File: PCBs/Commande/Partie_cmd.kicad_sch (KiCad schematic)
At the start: 74 parts, among them J1 Barrel_Jack, J10 Conn_01x02, J2 Conn_01x04_Socket, J3 Conn_01x04_Socket, J4 Conn_01x15, J6 Conn_01x04, J7 Conn_01x04, J9 Conn_01x02, U1 ESP32-S3-DEVKITC-1-N8R2, U2 BU18SD5WG-TL, U3 BU33SD5WG-TR, U4 XL1509-5.0

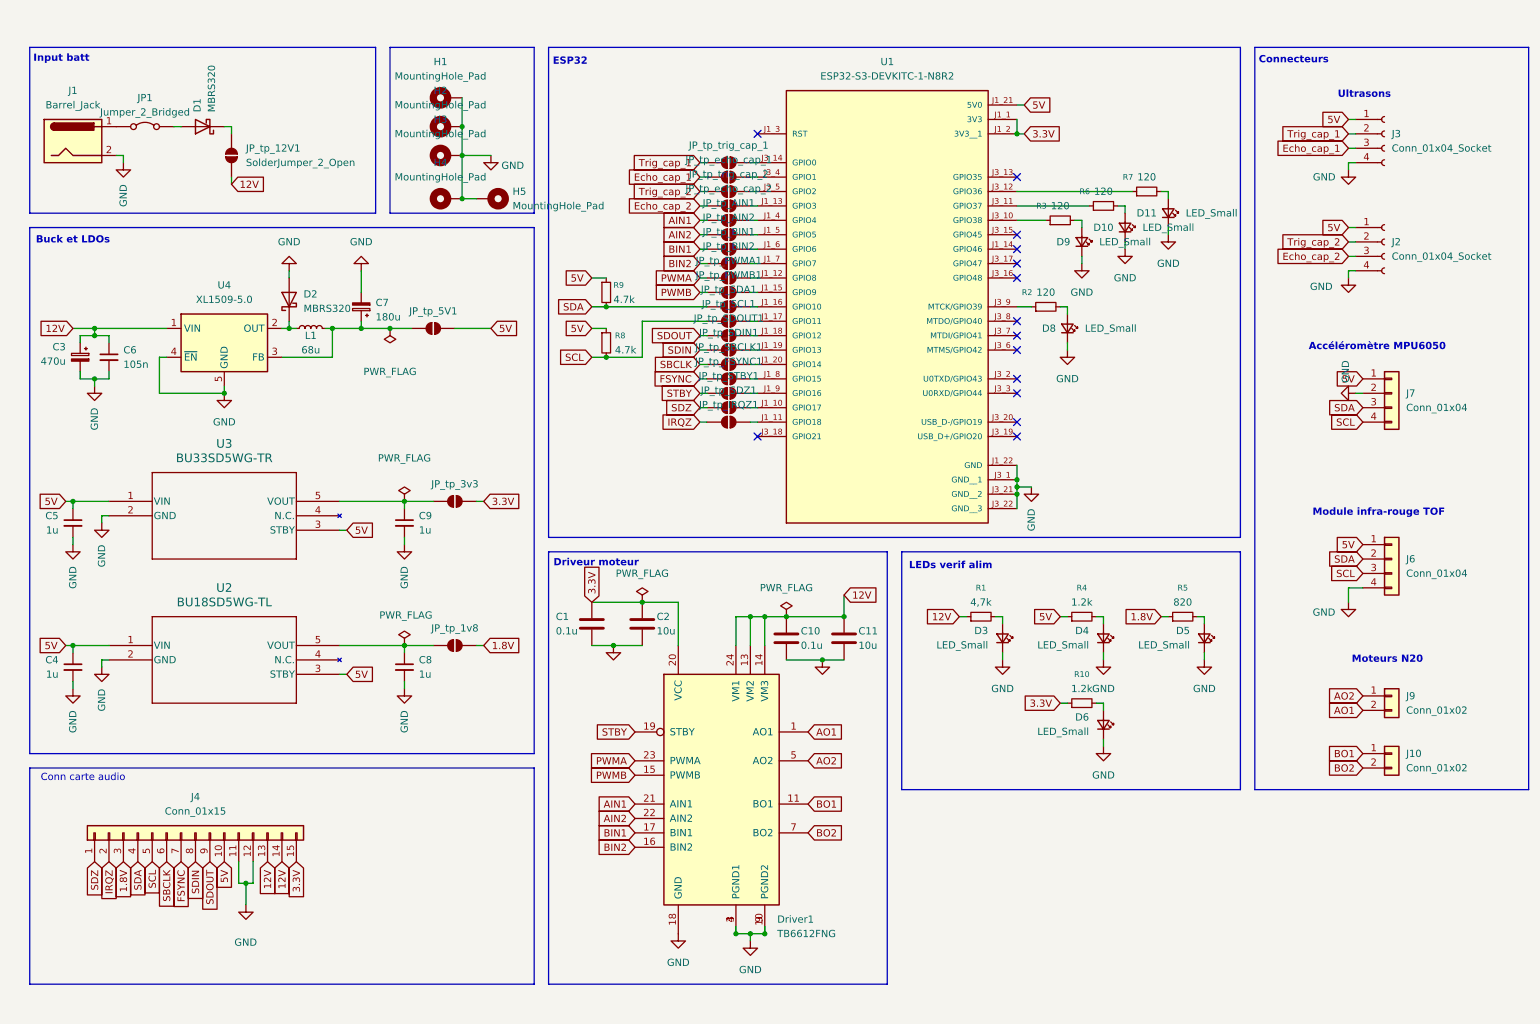
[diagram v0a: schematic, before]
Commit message: schema et pcb update
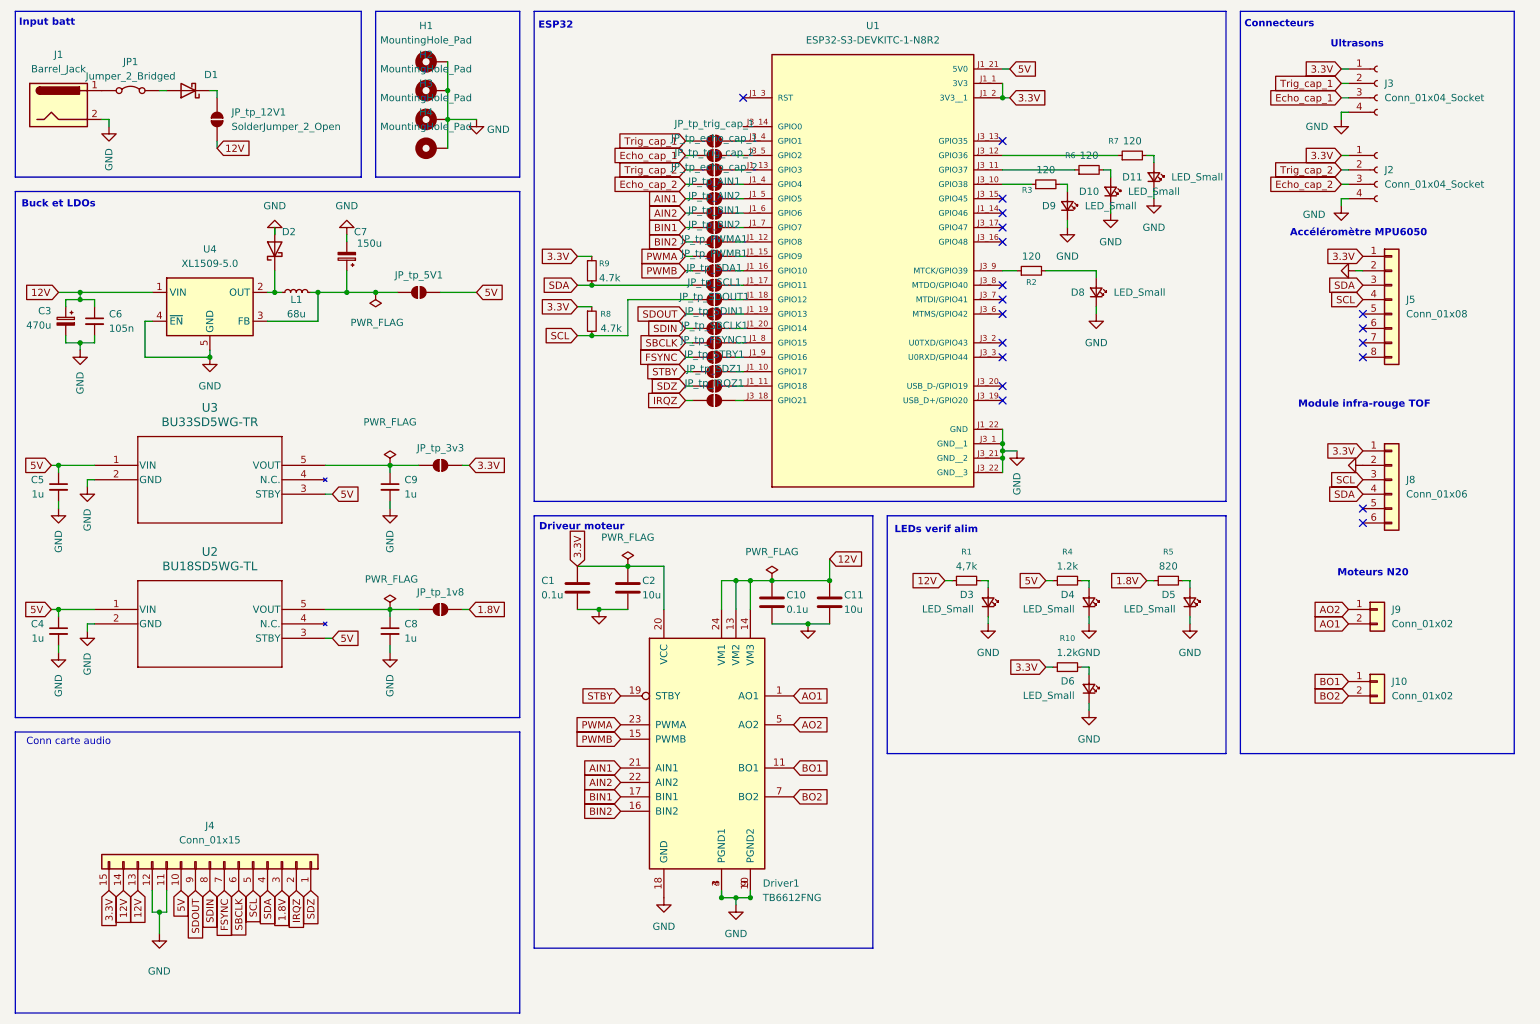
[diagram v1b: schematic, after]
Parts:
- removed H5: MountingHole_Pad, MountingHole:MountingHole_2.2mm_M2_DIN965_Pad, symbol Mechanical:MountingHole_Pad
- removed J6: Conn_01x04, Connector_PinSocket_1.00mm:PinSocket_1x04_P1.00mm_Vertical, symbol Connector_Generic:Conn_01x04
- removed J7: Conn_01x04, Connector_PinHeader_1.27mm:PinHeader_1x04_P1.27mm_Vertical, symbol Connector_Generic:Conn_01x04
- added J5: Conn_01x08, Connector_PinHeader_2.54mm:PinHeader_1x08_P2.54mm_Vertical, symbol Connector_Generic:Conn_01x08
- added J8: Conn_01x06, Connector_PinHeader_2.54mm:PinHeader_1x06_P2.54mm_Vertical, symbol Connector_Generic:Conn_01x06
- C3: footprint Capacitor_SMD:C_0603_1608Metric_Pad1.08x0.95mm_HandSolder -> Capacitor_SMD:CP_Elec_8x10.5
- C7: value 180u -> 150u; footprint Capacitor_SMD:C_0603_1608Metric_Pad1.08x0.95mm_HandSolder -> Capacitor_SMD:CP_Elec_6.3x7.7
- H4: footprint MountingHole:MountingHole_2.2mm_M2_DIN965_Pad -> MountingHole:MountingHole_2.5mm_Pad_Via
- J2, J3: footprint Connector_PinSocket_1.27mm:PinSocket_1x04_P1.27mm_Vertical -> Connector_PinHeader_2.54mm:PinHeader_1x04_P2.54mm_Vertical
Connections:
- net 3.3V: now also J2.1 (Pin_1), J3.1 (Pin_1), R8.1, R9.1, J5.1 (Pin_1), J8.1 (Pin_1)
- net 5V: no longer J2.1 (Pin_1), J3.1 (Pin_1), R8.1, R9.1
- net GND: now also J5.2 (Pin_2), J8.2 (Pin_2)
- net SCL: now also J5.4 (Pin_4), J8.3 (Pin_3)
- net SDA: now also J5.3 (Pin_3), J8.4 (Pin_4)
- net at JP_tp_SDZ1.2 (B): now also U1.J1_11 (GPIO18); no longer U1.J1_10 (GPIO17)
- net at JP_tp_IRQZ1.2 (B): now also U1.J3_18 (GPIO21); no longer U1.J1_11 (GPIO18)
- net at U1.J1_12 (GPIO8): now also JP_tp_BIN2.2 (B); no longer JP_tp_PWMA1.2 (B)
- net at U1.J1_13 (GPIO3): now also JP_tp_trig_cap_2.2 (B); no longer JP_tp_echo_cap_2.2 (B)
- net at U1.J1_15 (GPIO9): now also JP_tp_PWMA1.2 (B); no longer JP_tp_PWMB1.2 (B)
- net at U1.J1_16 (GPIO10): now also JP_tp_PWMB1.2 (B); no longer JP_tp_SDA1.2 (B)
- net at U1.J1_17 (GPIO11): now also JP_tp_SDA1.2 (B); no longer JP_tp_SCL1.2 (B)
- net at U1.J1_18 (GPIO12): now also JP_tp_SCL1.2 (B); no longer JP_tp_SDOUT1.2 (B)
- net at U1.J1_19 (GPIO13): now also JP_tp_SDOUT1.2 (B); no longer JP_tp_SDIN1.2 (B)
- net at U1.J1_20 (GPIO14): now also JP_tp_SDIN1.2 (B); no longer JP_tp_SBCLK1.2 (B)
- net at U1.J1_4 (GPIO4): now also JP_tp_echo_cap_2.2 (B); no longer JP_tp_AIN1.2 (B)
- net at U1.J1_5 (GPIO5): now also JP_tp_AIN1.2 (B); no longer JP_tp_AIN2.2 (B)
- net at U1.J1_6 (GPIO6): now also JP_tp_AIN2.2 (B); no longer JP_tp_BIN1.2 (B)
- net at U1.J1_7 (GPIO7): now also JP_tp_BIN1.2 (B); no longer JP_tp_BIN2.2 (B)
- net at U1.J1_8 (GPIO15): now also JP_tp_SBCLK1.2 (B); no longer JP_tp_FSYNC1.2 (B)
- net at JP_tp_STBY1.2 (B): now also U1.J1_10 (GPIO17); no longer U1.J1_9 (GPIO16)
- net at U1.J3_14 (GPIO0): no longer JP_tp_trig_cap_1.2 (B)
- net at U1.J3_4 (GPIO1): now also JP_tp_trig_cap_1.2 (B); no longer JP_tp_echo_cap_1.2 (B)
- net at U1.J3_5 (GPIO2): now also JP_tp_echo_cap_1.2 (B); no longer JP_tp_trig_cap_2.2 (B)
- new net: JP_tp_FSYNC1.2 (B), U1.J1_9 (GPIO16)
- no-connect marks 14 -> 19
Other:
- moved on the sheet: C1, C10, C11, C2, C3, C4, C5, C6, C7, C8, C9, D1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

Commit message: pcbss
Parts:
- J1: footprint Connector_BarrelJack:BarrelJack_Wuerth_694108106102_2.5x5.5mm -> BarrelJack (PPZ):CONN3_06105102_WRE
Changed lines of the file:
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@@
 			)
 		)
-		(property "Footprint" "Connector_BarrelJack:BarrelJack_Wuerth_694108106102_2.5x5.5mm"
+		(property "Footprint" "BarrelJack (PPZ):CONN3_06105102_WRE"
 			(at 25.4 34.036 0)
 			(effects

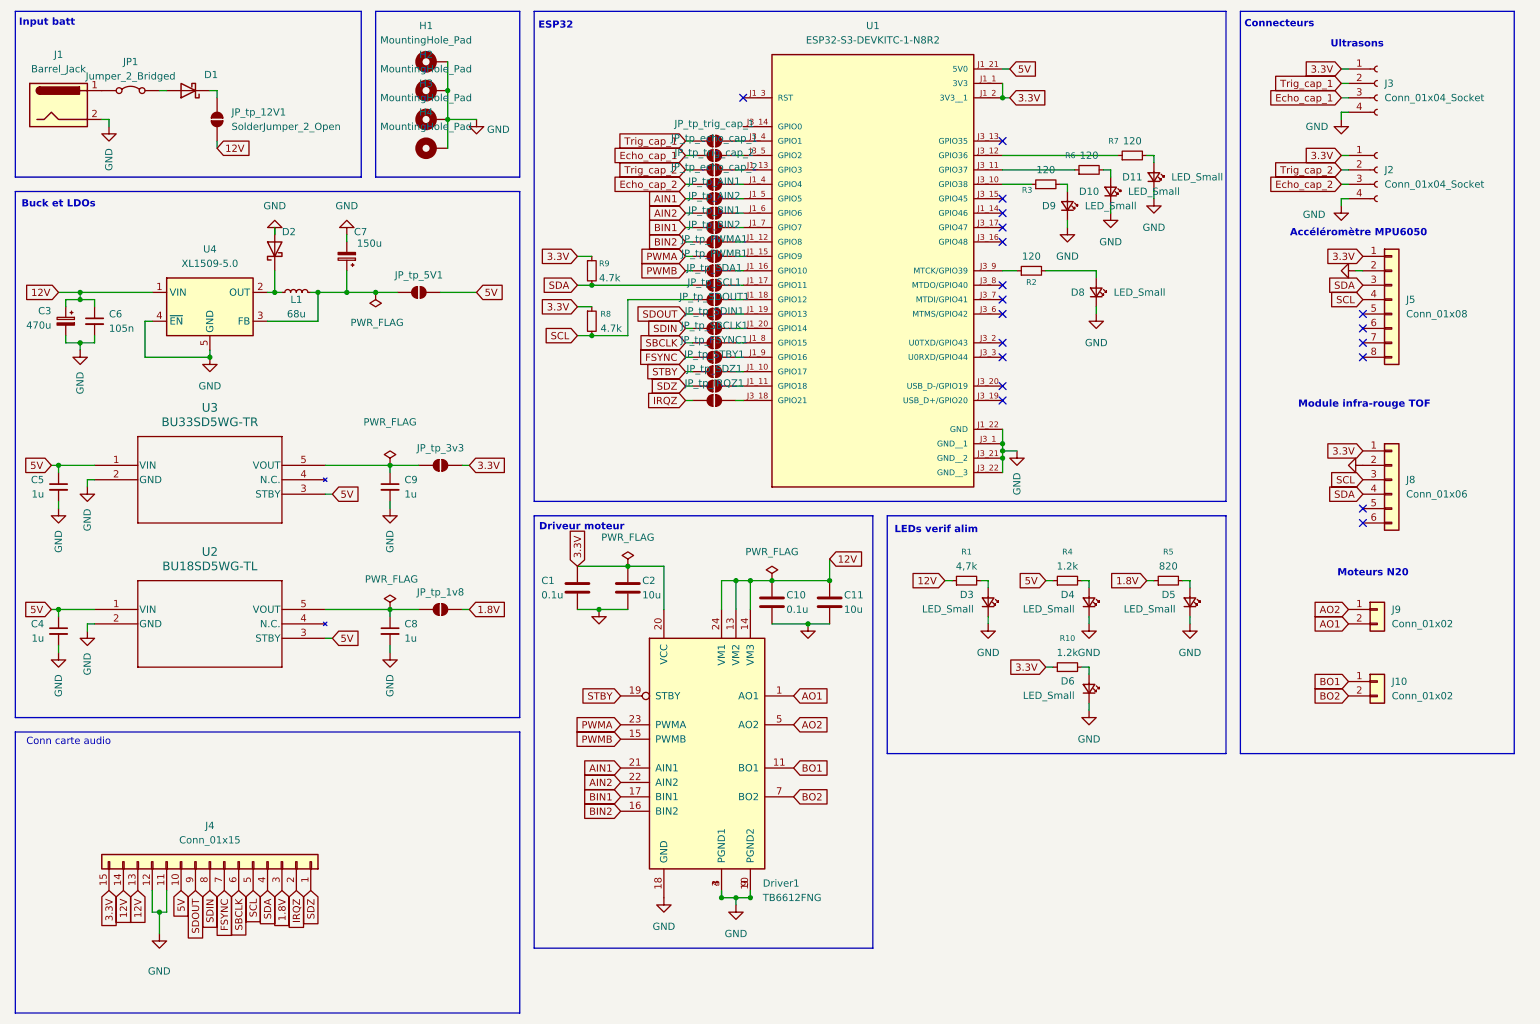
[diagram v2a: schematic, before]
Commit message: New pcb avec des erreurs
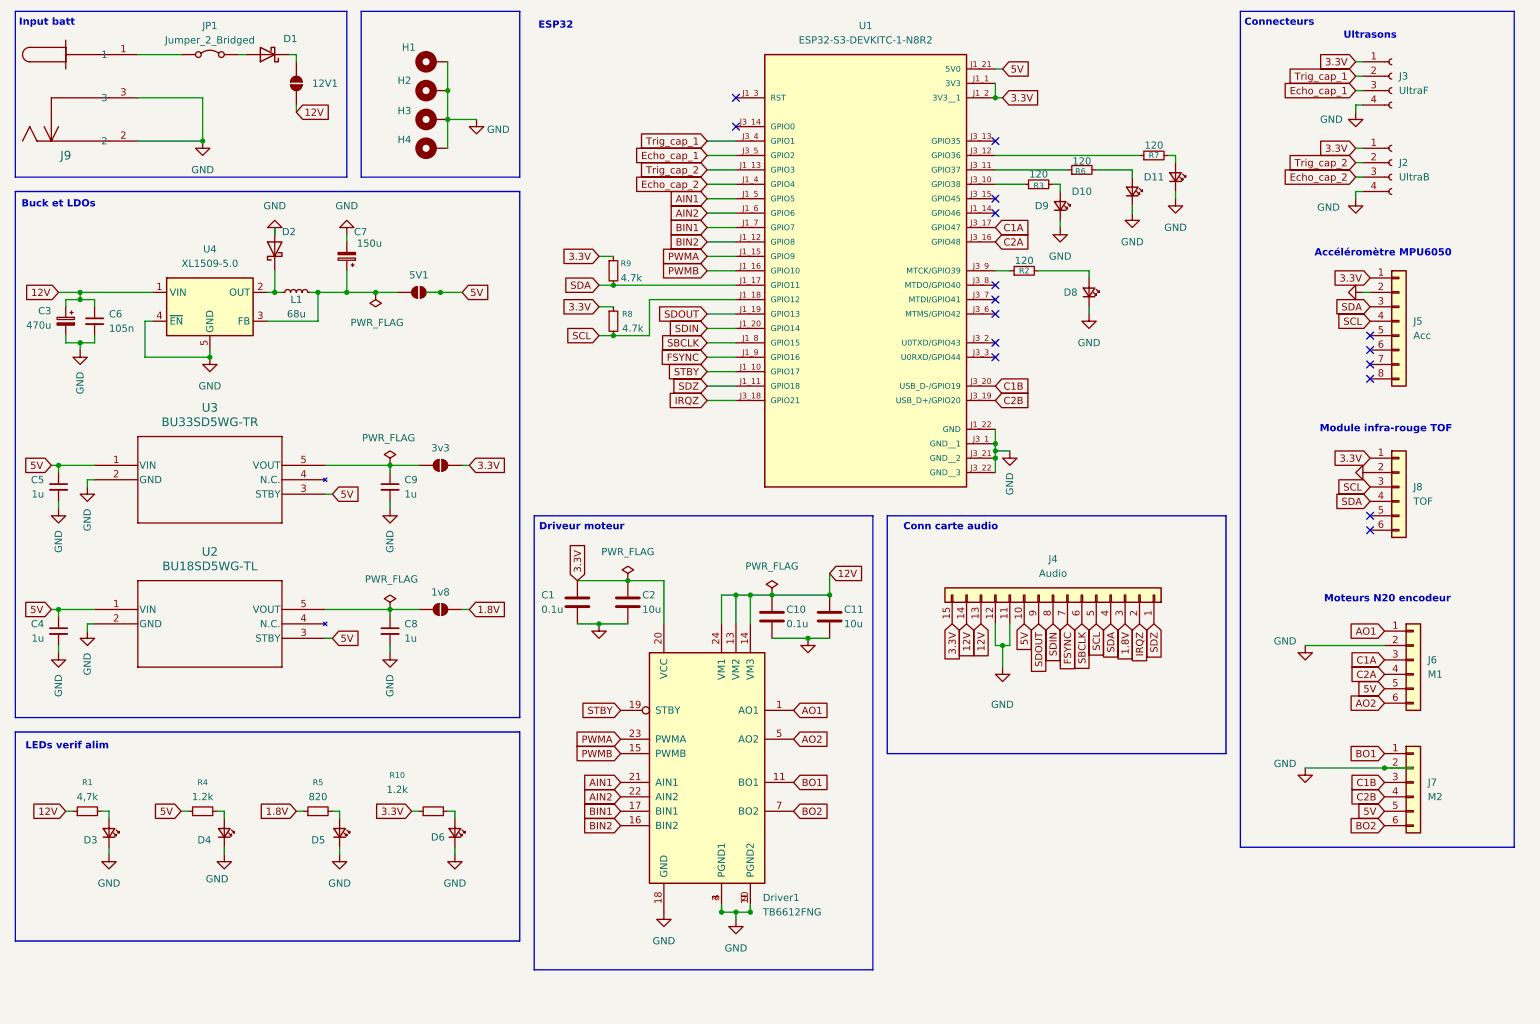
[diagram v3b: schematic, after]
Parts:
- removed J1: Barrel_Jack, BarrelJack (PPZ):CONN3_06105102_WRE, symbol Connector:Barrel_Jack
- removed J10, J9: Conn_01x02, Connector_JST:JST_XH_B2B-XH-A_1x02_P2.50mm_Vertical, symbol Connector_Generic:Conn_01x02
- removed JP_tp_AIN1, JP_tp_AIN2, JP_tp_BIN1, JP_tp_BIN2, JP_tp_FSYNC1, JP_tp_IRQZ1, JP_tp_PWMA1, JP_tp_PWMB1, JP_tp_SBCLK1, JP_tp_SCL1, JP_tp_SDA1, JP_tp_SDIN1, JP_tp_SDOUT1, JP_tp_SDZ1, JP_tp_STBY1, JP_tp_echo_cap_1, JP_tp_echo_cap_2, JP_tp_trig_cap_1, JP_tp_trig_cap_2: SolderJumper_2_Open, Jumper:SolderJumper-2_P1.3mm_Open_TrianglePad1.0x1.5mm, symbol Jumper:SolderJumper_2_Open
- added J6: M1, Connector_JST:JST_PH_B6B-PH-K_1x06_P2.00mm_Vertical, symbol Connector_Generic:Conn_01x06
- added J7: M2, Connector_JST:JST_PH_B6B-PH-K_1x06_P2.00mm_Vertical, symbol Connector_Generic:Conn_01x06
- added J9: 694106105102, Jack (PPZ):CONN3_06105102_WRE, symbol Jack (PPZ):694106105102
- J2: value Conn_01x04_Socket -> UltraB
- J3: value Conn_01x04_Socket -> UltraF
- J4: value Conn_01x15 -> Audio
- J5: value Conn_01x08 -> Acc
- J8: value Conn_01x06 -> TOF
- renumbered JP_tp_12V1 to 12V1, JP_tp_1v8 to 1v8, JP_tp_3v3 to 3v3, JP_tp_5V1 to 5V1
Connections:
- net 5V: now also J6.5 (Pin_5), J7.5 (Pin_5)
- net AIN1: now also U1.J1_5 (GPIO5)
- net AIN2: now also U1.J1_6 (GPIO6)
- net AO1: now also J6.1 (Pin_1)
- net AO2: now also J6.6 (Pin_6)
- net BIN1: now also U1.J1_7 (GPIO7)
- net BIN2: now also U1.J1_12 (GPIO8)
- net BO1: now also J7.1 (Pin_1)
- net BO2: now also J7.6 (Pin_6)
- net Echo_cap_1: now also U1.J3_5 (GPIO2)
- net Echo_cap_2: now also U1.J1_4 (GPIO4)
- net FSYNC: now also U1.J1_9 (GPIO16)
- net GND: now also J6.2 (Pin_2), J7.2 (Pin_2), J9.2, J9.3
- net IRQZ: now also U1.J3_18 (GPIO21)
- net PWMA: now also U1.J1_15 (GPIO9)
- net PWMB: now also U1.J1_16 (GPIO10)
- net SBCLK: now also U1.J1_8 (GPIO15)
- net SCL: now also U1.J1_18 (GPIO12)
- net SDA: now also U1.J1_17 (GPIO11)
- net SDIN: now also U1.J1_20 (GPIO14)
- net SDOUT: now also U1.J1_19 (GPIO13)
- net SDZ: now also U1.J1_11 (GPIO18)
- net STBY: now also U1.J1_10 (GPIO17)
- net Trig_cap_1: now also U1.J3_4 (GPIO1)
- net Trig_cap_2: now also U1.J1_13 (GPIO3)
- net at JP1.1 (A): now also J9.1
- net C2A: now reaches U1.J3_16 (GPIO48)
- net C2A: now also J6.4 (Pin_4)
- net C1A: now reaches U1.J3_17 (GPIO47)
- net C1A: now also J6.3 (Pin_3)
- net C2B: now reaches U1.J3_19 (USB_D+/GPIO20)
- net C2B: now also J7.4 (Pin_4)
- net C1B: now reaches U1.J3_20 (USB_D-/GPIO19)
- net C1B: now also J7.3 (Pin_3)
- no-connect marks 19 -> 16
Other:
- note added: "Moteurs N20 encodeur"
- note removed: "Moteurs N20"
- moved on the sheet: 12V1, C1, C10, C11, C2, D1, D10, D11, D3, D4, D5, D6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

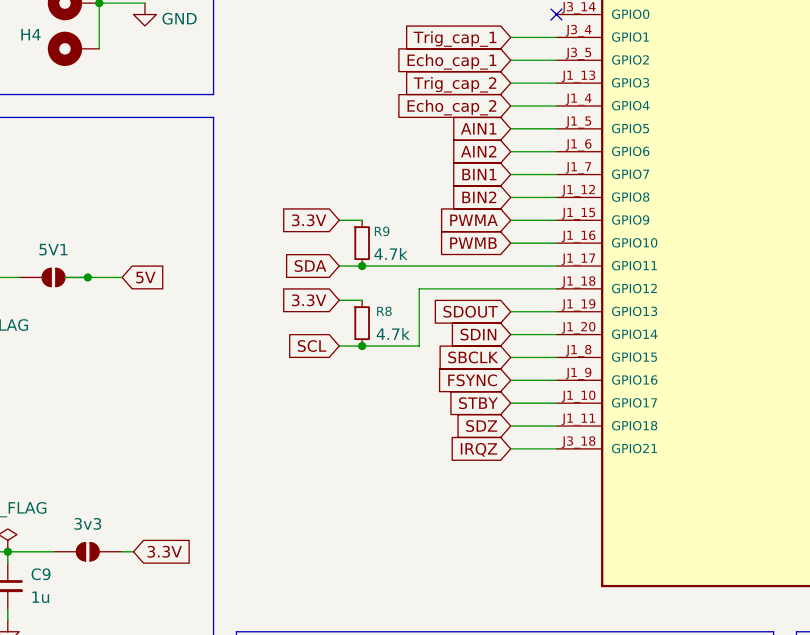
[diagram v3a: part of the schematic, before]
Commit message: edit pcb
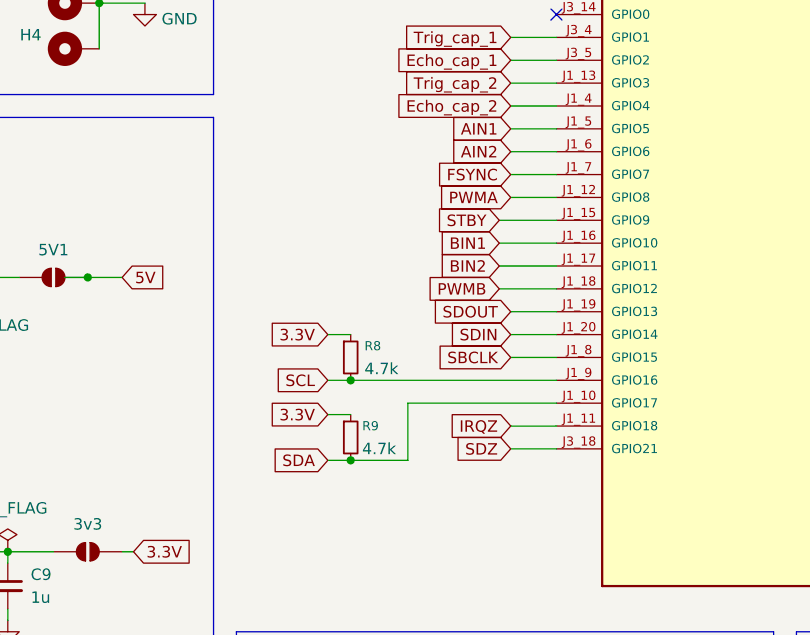
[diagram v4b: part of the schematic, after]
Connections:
- net BIN1: now also U1.J1_16 (GPIO10); no longer U1.J1_7 (GPIO7)
- net BIN2: now also U1.J1_17 (GPIO11); no longer U1.J1_12 (GPIO8)
- net FSYNC: now also U1.J1_7 (GPIO7); no longer U1.J1_9 (GPIO16)
- net IRQZ: now also U1.J1_11 (GPIO18); no longer U1.J3_18 (GPIO21)
- net PWMA: now also U1.J1_12 (GPIO8); no longer U1.J1_15 (GPIO9)
- net PWMB: now also U1.J1_18 (GPIO12); no longer U1.J1_16 (GPIO10)
- net SCL: now also U1.J1_9 (GPIO16); no longer U1.J1_18 (GPIO12)
- net SDA: now also U1.J1_10 (GPIO17); no longer U1.J1_17 (GPIO11)
- net SDZ: now also U1.J3_18 (GPIO21); no longer U1.J1_11 (GPIO18)
- net STBY: now also U1.J1_15 (GPIO9); no longer U1.J1_10 (GPIO17)
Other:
- moved on the sheet: R8, R9
